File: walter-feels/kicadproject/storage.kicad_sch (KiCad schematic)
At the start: 4 parts, among them J1 693072010801, U13 CM1624-08DE

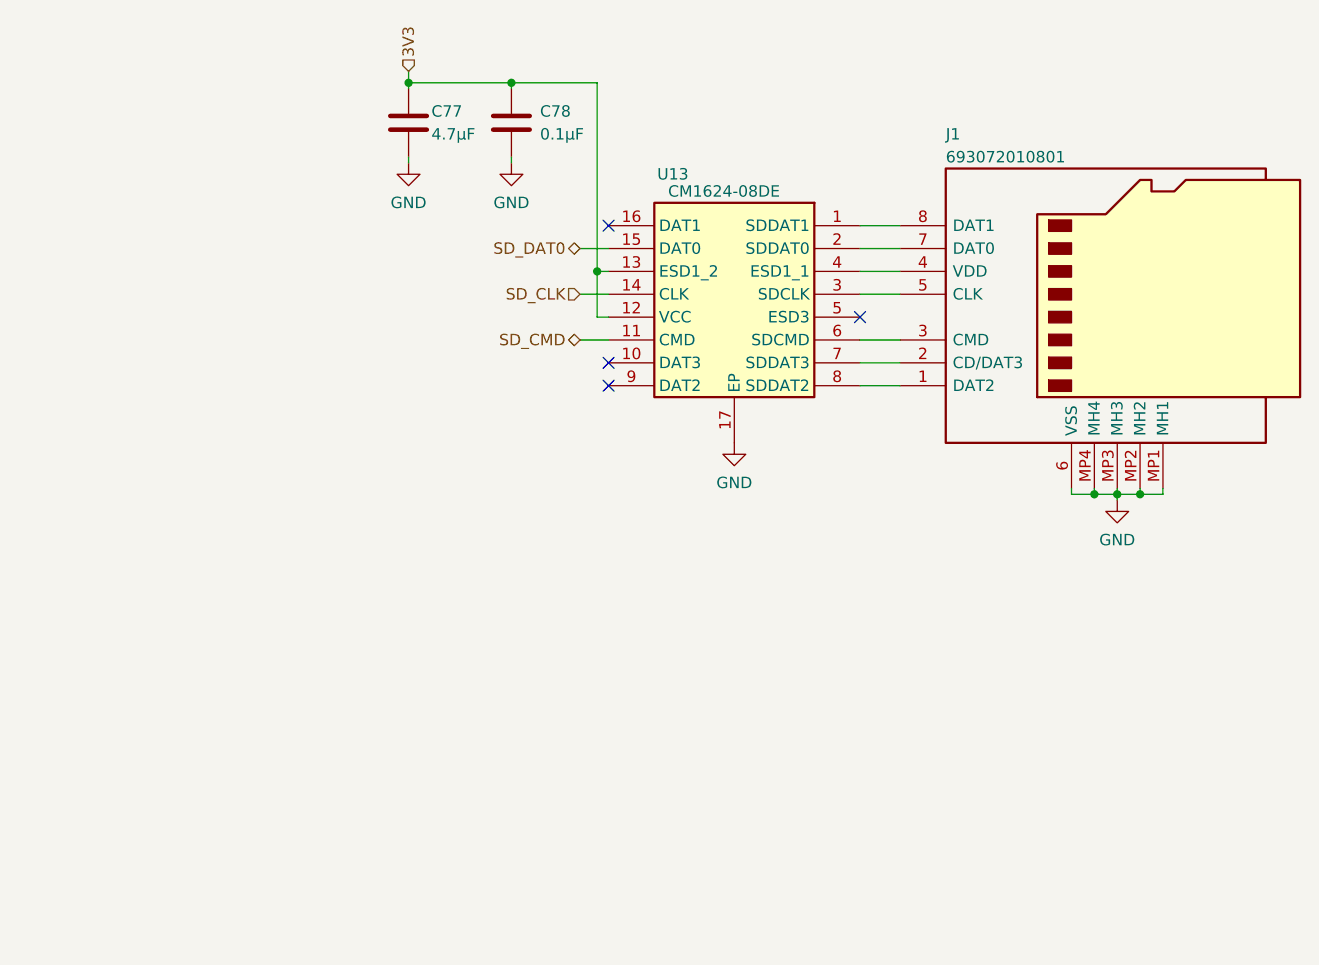
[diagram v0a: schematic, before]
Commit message: Updated Walter Feels project to version 2.6
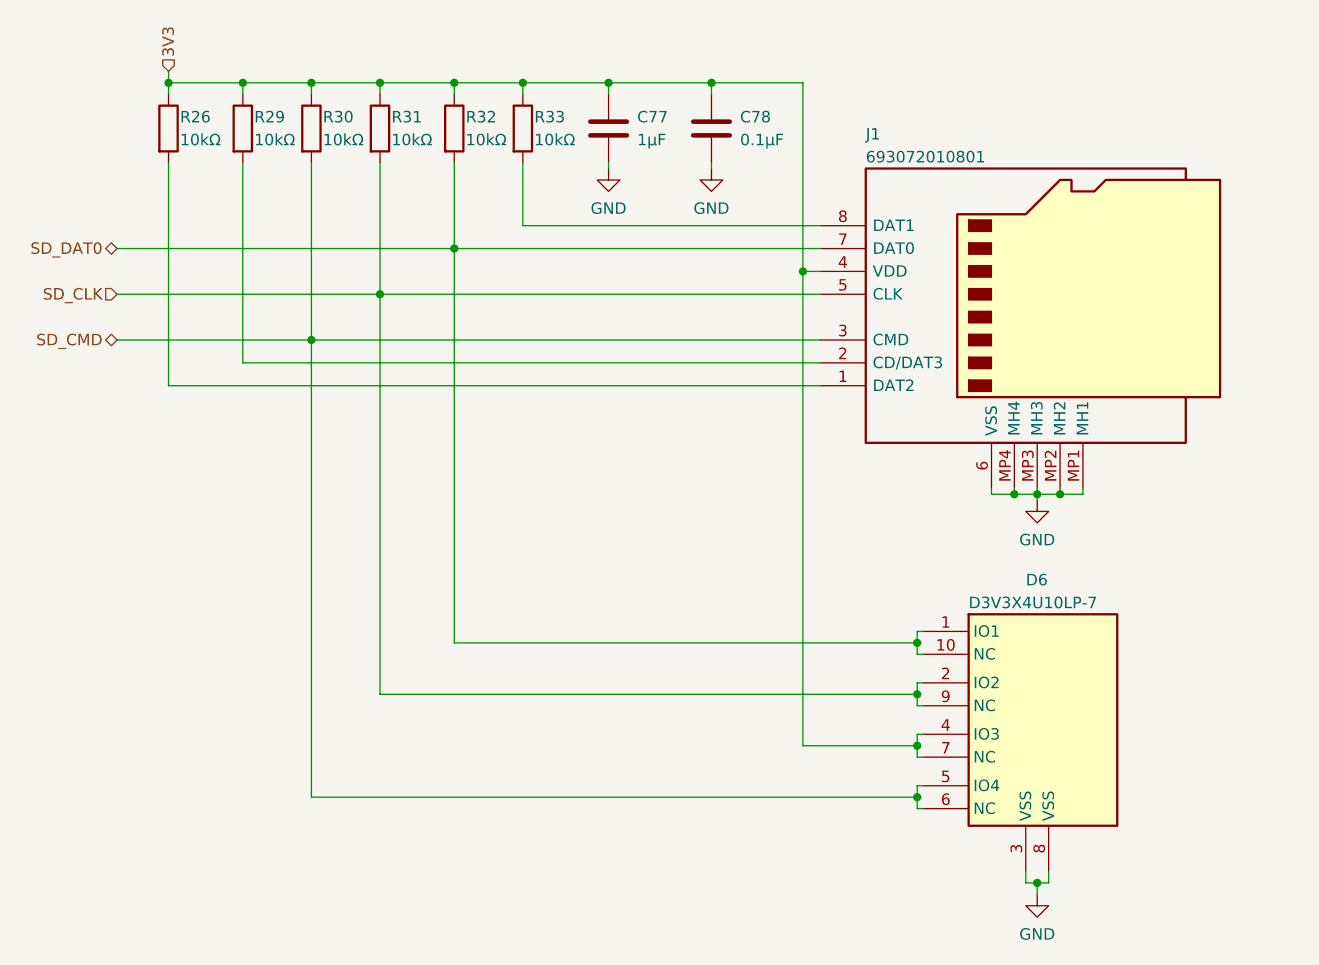
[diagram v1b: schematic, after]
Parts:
- removed U13: CM1624-08DE, LIB_CM1624-08DE:SON40P135X330X55-17N, symbol CM1624-08DE:CM1624-08DE
- added D6: D3V3X4U10LP-7, D3V3X4U10LP-7:D3V3X4U10LP7, symbol D3V3X4U10LP-7:D3V3X4U10LP-7
- added R26, R29, R30, R31, R32, R33: 10kΩ, Resistor_SMD:R_0603_1608Metric, symbol Device:R
- C77: value 4.7μF -> 1μF; JLCPCB C19666 -> C15849
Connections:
- net 3V3: now also J1.4 (VDD), D6.4 (IO3), D6.7 (NC), R26.1, R29.1, R30.1, R31.1, R32.1, R33.1
- net GND: now also D6.3 (VSS), D6.8 (VSS)
- net SD_CLK: now also J1.5 (CLK), D6.2 (IO2), D6.9 (NC), R31.2
- net SD_CMD: now also J1.3 (CMD), D6.5 (IO4), D6.6 (NC), R30.2
- net SD_DAT0: now also J1.7 (DAT0), D6.1 (IO1), D6.10 (NC), R32.2
- net at J1.1 (DAT2): now also R26.2
- net at J1.2 (CD/DAT3): now also R29.2
- net at J1.8 (DAT1): now also R33.2
- no-connect marks 4 -> 0
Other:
- moved on the sheet: C78, J1
